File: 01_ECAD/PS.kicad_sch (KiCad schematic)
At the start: 76 parts, among them J1 B2P3-VH(LF)(SN), J2 B4P-VH(LF)(SN), Q1 IXFH20N100P, SW1 NE18 2A EE 6AMP, U1 UCC28600, U2 CNY17-1, U3 TL431DBZ

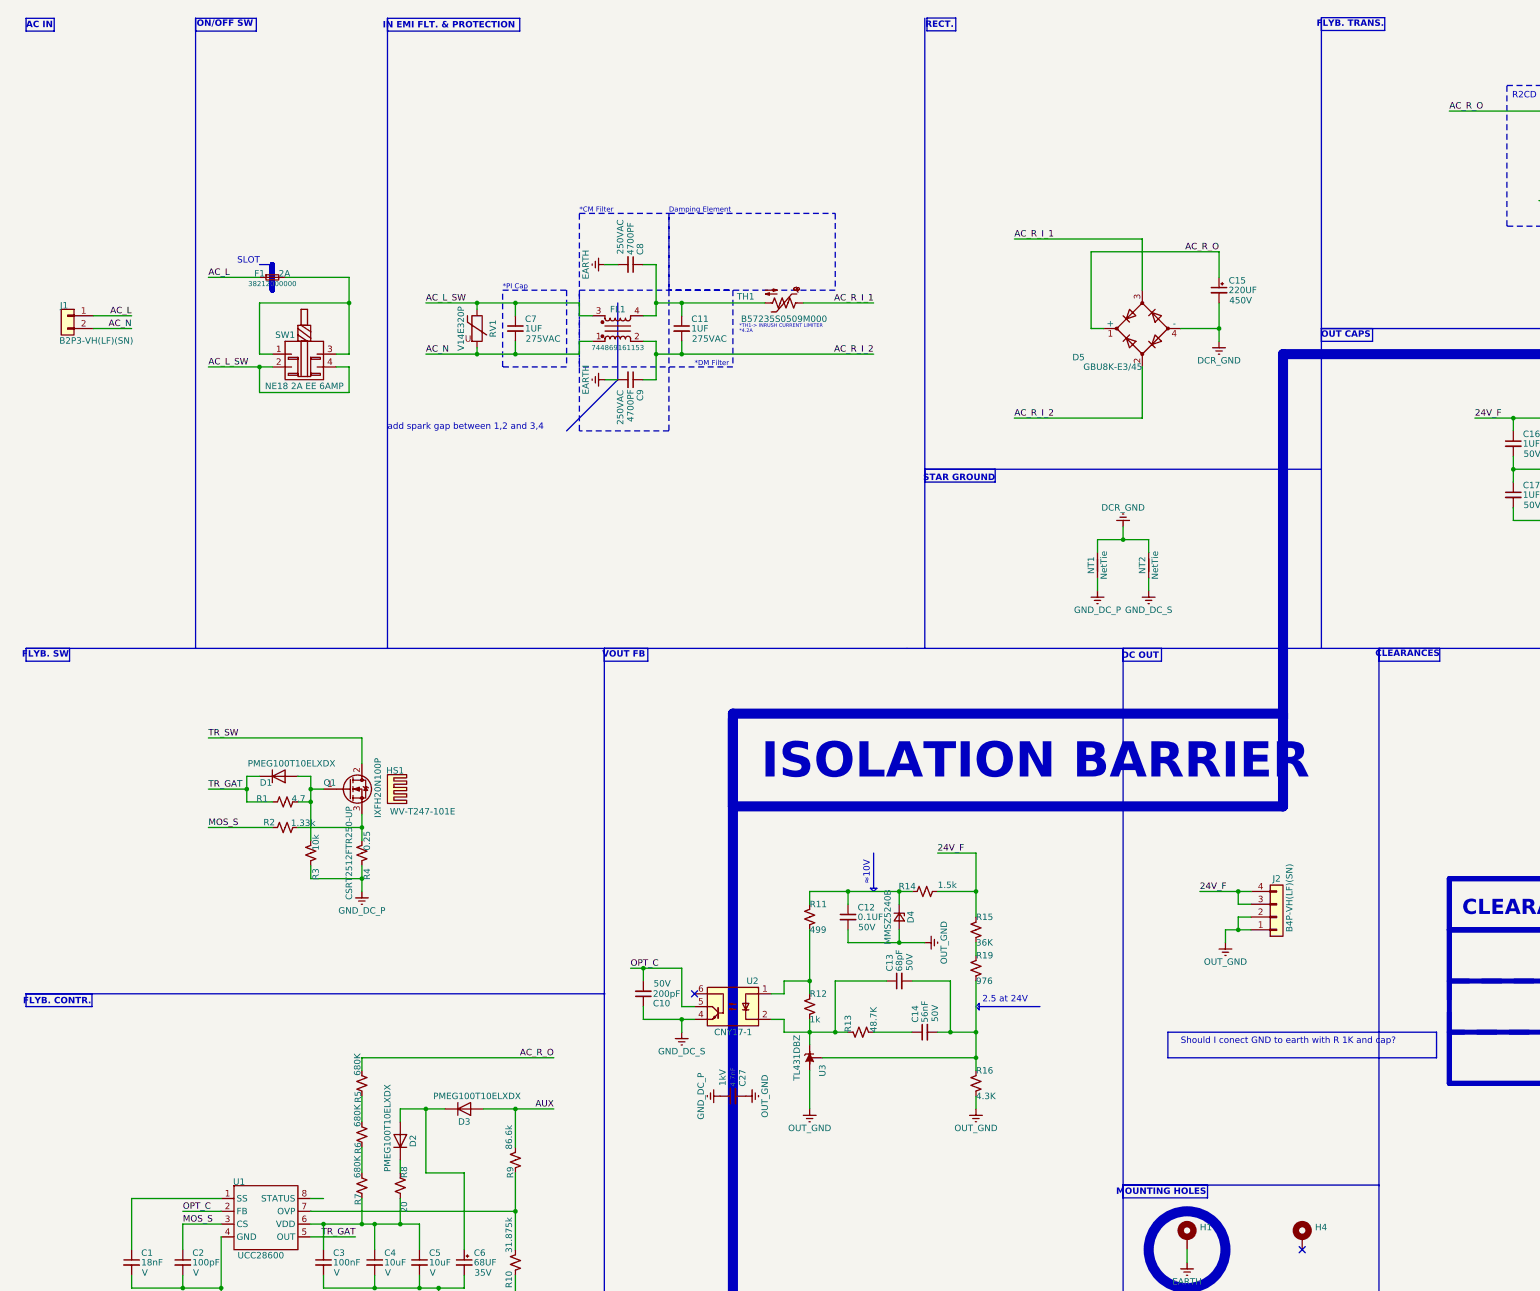
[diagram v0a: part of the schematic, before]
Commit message: Update.
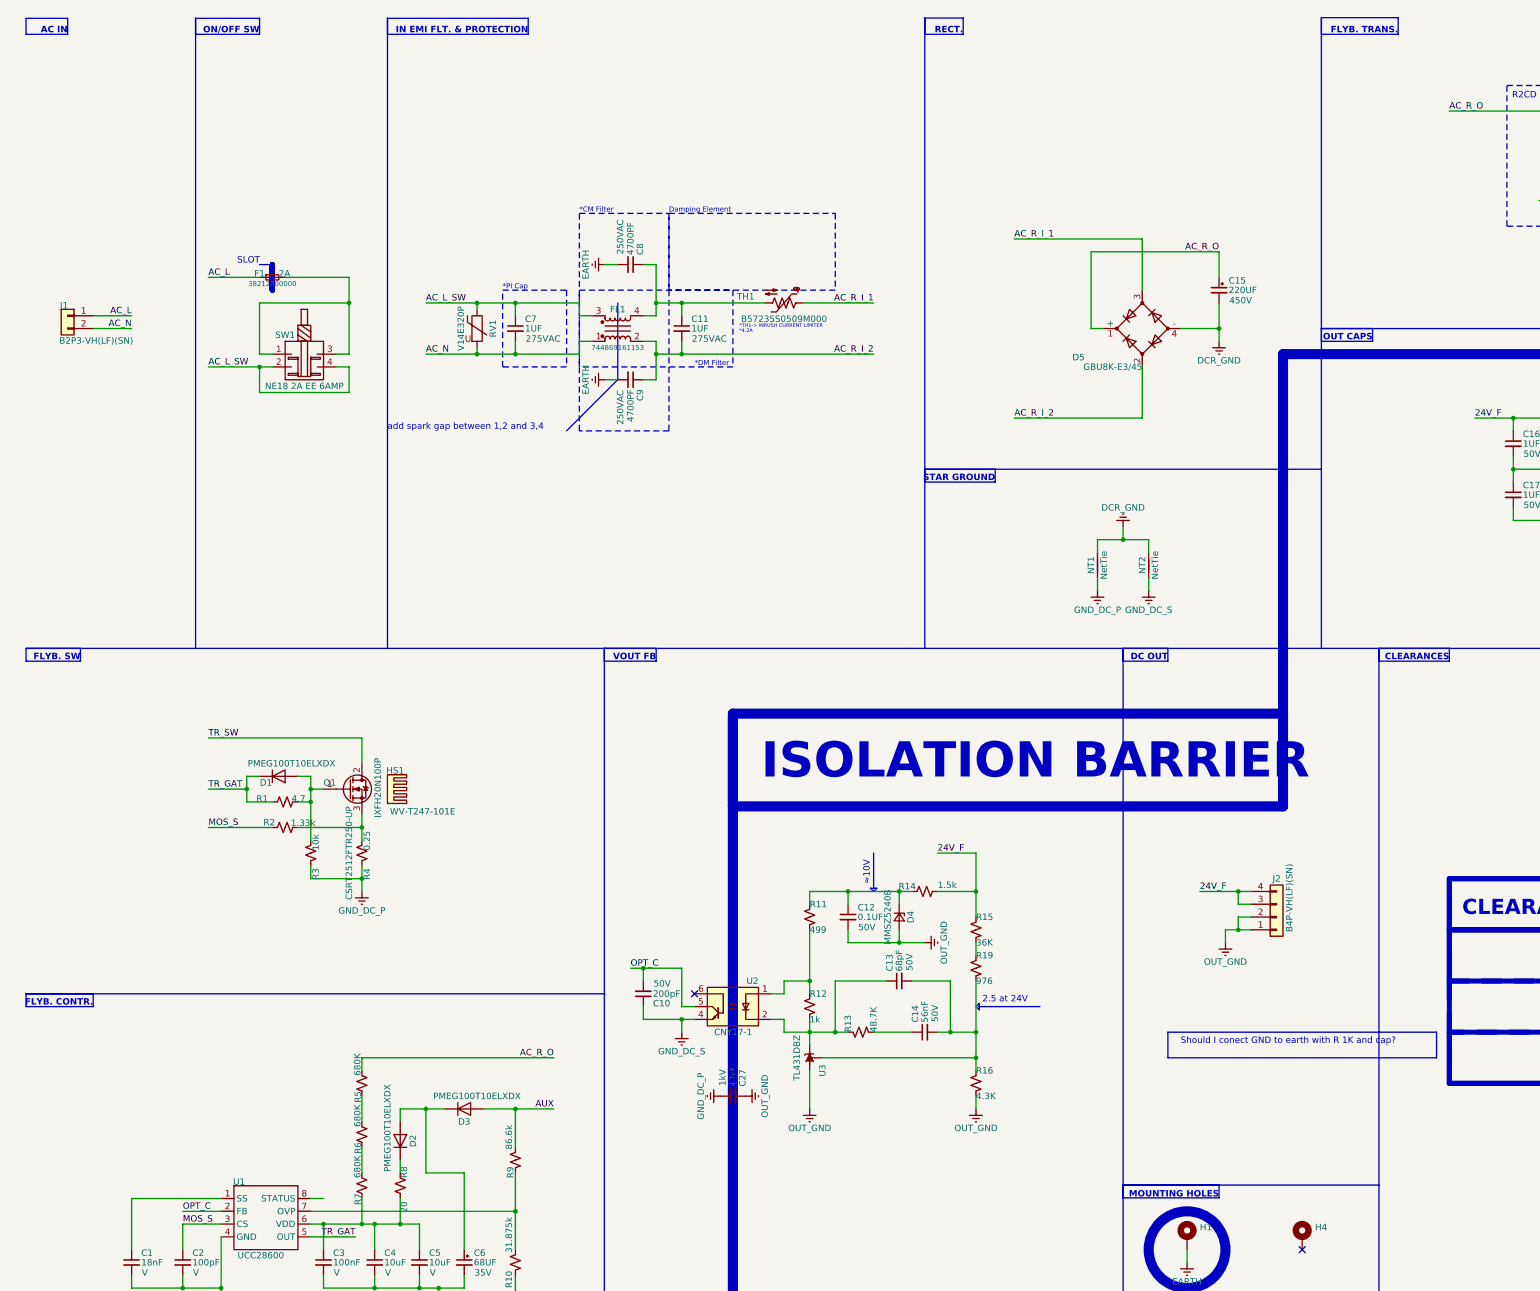
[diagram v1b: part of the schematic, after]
